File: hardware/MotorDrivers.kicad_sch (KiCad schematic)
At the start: 8 parts, among them M1 M1_CONN, M2 M2_CONN, M3 M3_CONN, M4 M4_CONN, U103 STSPIN240, U104 STSPIN240, U105 STSPIN240, U106 STSPIN240

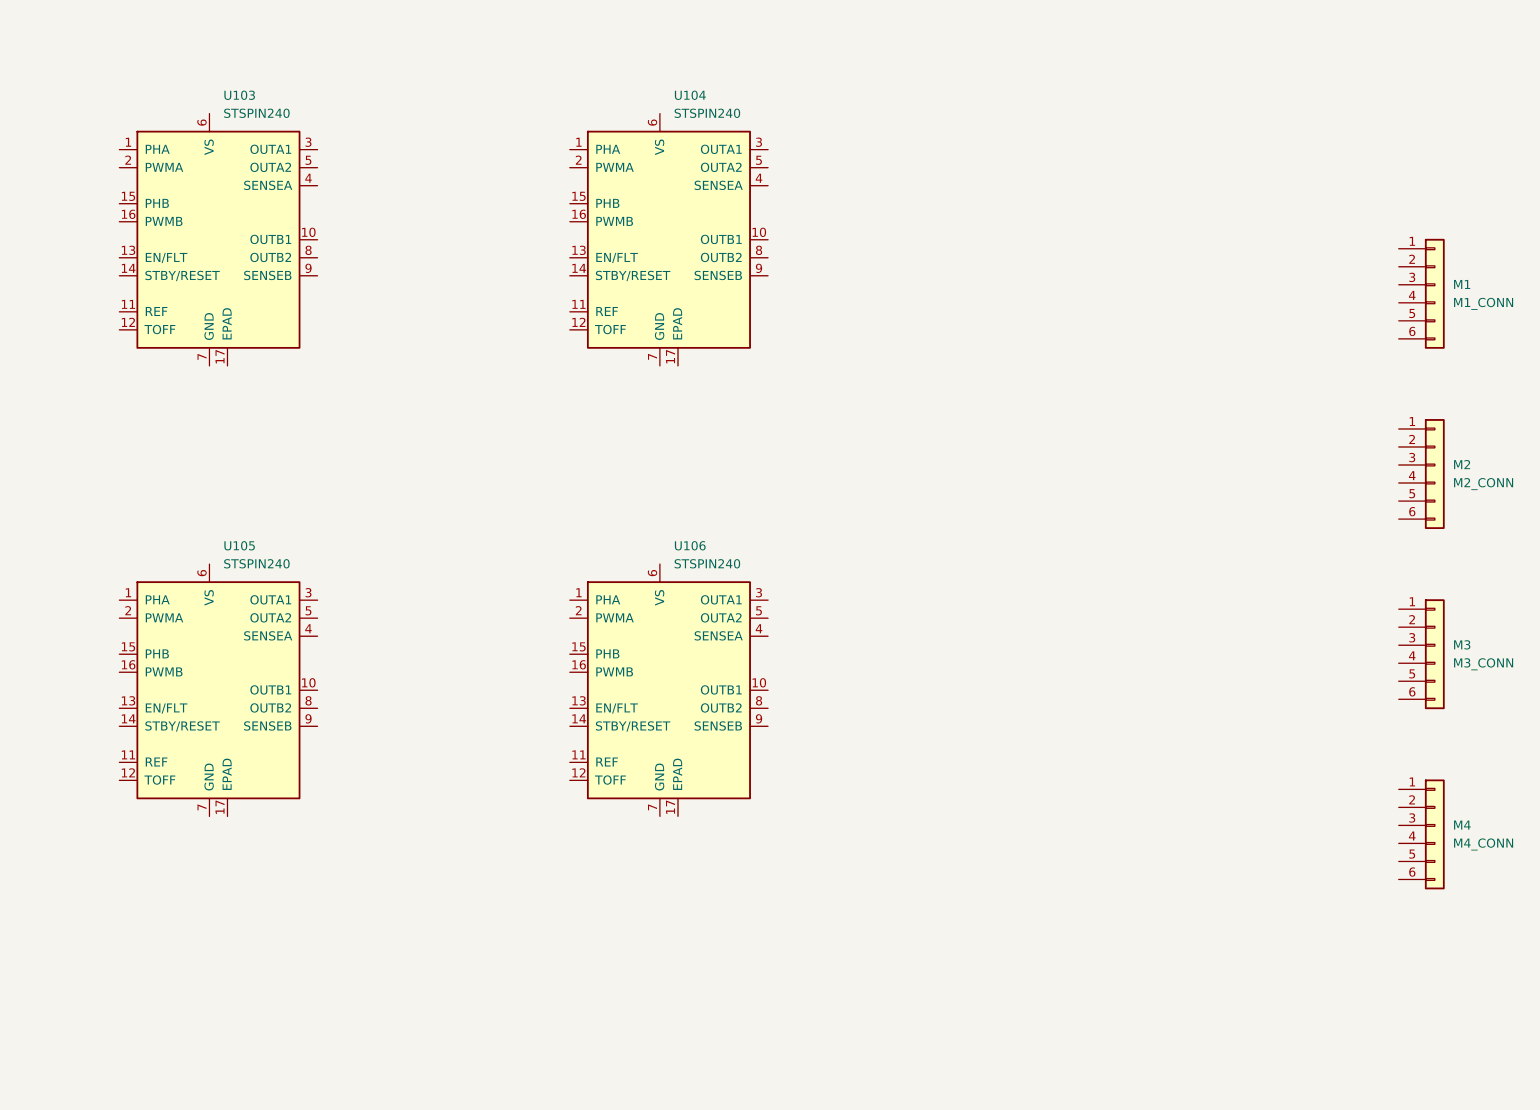
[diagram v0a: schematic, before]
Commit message: asdf
Signed-off-by: Connor Rigby <connorr@hey.com>
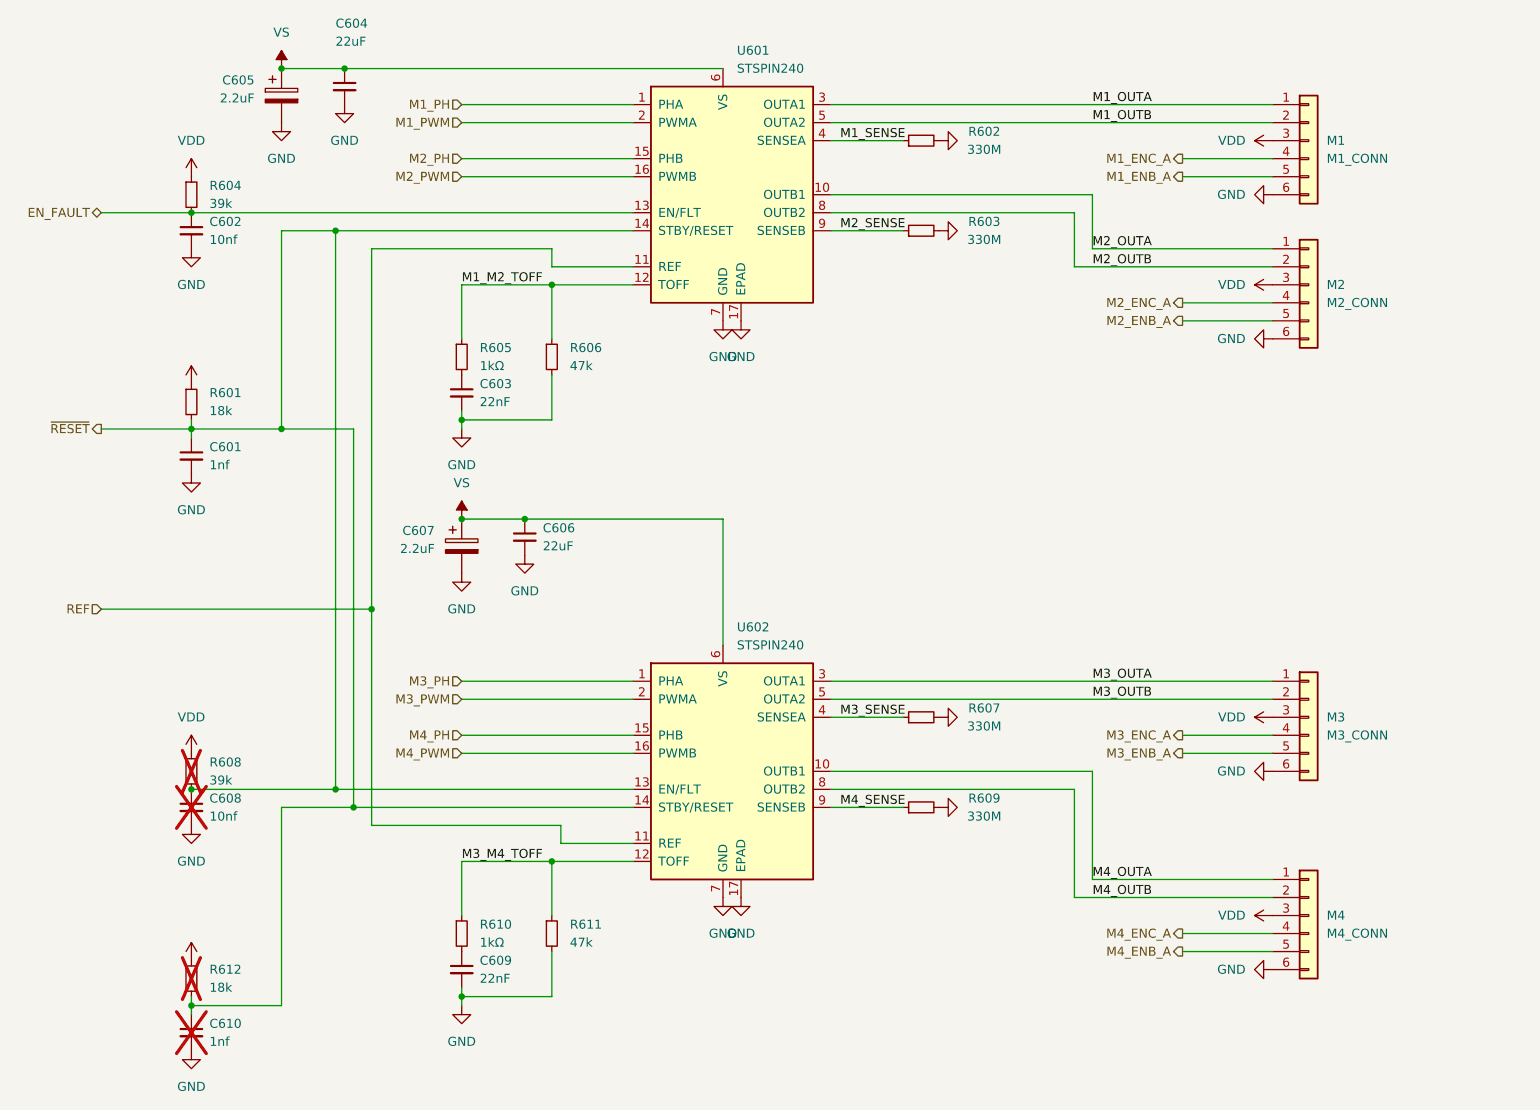
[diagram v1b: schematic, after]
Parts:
- removed U103, U104, U105, U106: STSPIN240, Package_DFN_QFN:VQFN-16-1EP_3x3mm_P0.5mm_EP1.8x1.8mm, symbol Driver_Motor:STSPIN240
- added C601, C610: C_0402_1nf_X7R, Capacitor_SMD:C_0402_1005Metric, symbol LCSC_Capacitor:C_0402_1nf_X7R
- added C602, C608: C_0402_10n_C0G, Capacitor_SMD:C_0402_1005Metric, symbol LCSC_Capacitor:C_0402_10n_C0G
- added C603, C609: C_0402_DNP, Capacitor_SMD:C_0402_1005Metric, symbol LCSC_Capacitor:C_0402_DNP
- added C604, C606: C_805_DNP, Capacitor_SMD:C_0805_2012Metric, symbol LCSC_Capacitor:C_805_DNP
- added C605, C607: 2.2uF, Capacitor_SMD:CP_Elec_5x3, symbol Device:C_Polarized
- added R601, R612: 18k, Resistor_SMD:R_0402_1005Metric, symbol LCSC_Resistor:R_0402_DNP
- added R602, R603, R607, R609: 330M, Resistor_SMD:R_0805_2012Metric, symbol Device:R_Small
- added R604, R608: 39k, Resistor_SMD:R_0402_1005Metric, symbol LCSC_Resistor:R_0402_DNP
- added R605, R610: R_0402_1k, Resistor_SMD:R_0402_1005Metric, symbol LCSC_Resistor:R_0402_1k
- added R606, R611: 47k, Resistor_SMD:R_0402_1005Metric, symbol LCSC_Resistor:R_0402_DNP
- added U601, U602: STSPIN240, Package_DFN_QFN:VQFN-16-1EP_3x3mm_P0.5mm_EP1.8x1.8mm, symbol Driver_Motor:STSPIN240
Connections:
- net M1_OUTA: now reaches M1.1 (Pin_1)
- net M1_OUTA: now also U601.3 (OUTA1)
- net M1_OUTB: now reaches M1.2 (Pin_2)
- net M1_OUTB: now also U601.5 (OUTA2)
- net VDD: now reaches M1.3 (Pin_3)
- net VDD: now also M2.3 (Pin_3), M3.3 (Pin_3), M4.3 (Pin_3), R601.1, R604.1, R608.1, R612.1
- net M1_ENC_A: now reaches M1.4 (Pin_4)
- net M1_ENB_A: now reaches M1.5 (Pin_5)
- net GND: now reaches M1.6 (Pin_6)
- net GND: now also M2.6 (Pin_6), M3.6 (Pin_6), M4.6 (Pin_6), C601.2, C602.2, C603.2, C604.2, C605.2, C606.2, C607.2, C608.2, C609.2, C610.2, R602.2, R603.2, R606.2, R607.2, R609.2, R611.2, U601.17 (EPAD), U601.7 (GND), U602.17 (EPAD), U602.7 (GND)
- net M4_OUTA: now reaches M4.1 (Pin_1)
- net M4_OUTA: now also U602.10 (OUTB1)
- net M4_OUTB: now reaches M4.2 (Pin_2)
- net M4_OUTB: now also U602.8 (OUTB2)
- net M4_ENC_A: now reaches M4.4 (Pin_4)
- net M4_ENB_A: now reaches M4.5 (Pin_5)
- net M2_OUTA: now reaches M2.1 (Pin_1)
- net M2_OUTA: now also U601.10 (OUTB1)
- net M2_OUTB: now reaches M2.2 (Pin_2)
- net M2_OUTB: now also U601.8 (OUTB2)
- net M2_ENC_A: now reaches M2.4 (Pin_4)
- net M2_ENB_A: now reaches M2.5 (Pin_5)
- net M3_OUTA: now reaches M3.1 (Pin_1)
- net M3_OUTA: now also U602.3 (OUTA1)
- net M3_OUTB: now reaches M3.2 (Pin_2)
- net M3_OUTB: now also U602.5 (OUTA2)
- net M3_ENC_A: now reaches M3.4 (Pin_4)
- net M3_ENB_A: now reaches M3.5 (Pin_5)
- new net: C603.1, R605.2
- new net: C609.1, R610.2
- new net EN_FAULT: C602.1, R604.2, U601.13 (EN/FLT)
- new net M1_M2_TOFF: R605.1, R606.1, U601.12 (TOFF)
- new net M1_PH: U601.1 (PHA)
- new net M1_PWM: U601.2 (PWMA)
- new net M1_SENSE: R602.1, U601.4 (SENSEA)
- new net M2_PH: U601.15 (PHB)
- new net M2_PWM: U601.16 (PWMB)
- new net M2_SENSE: R603.1, U601.9 (SENSEB)
- new net M3_M4_TOFF: R610.1, R611.1, U602.12 (TOFF)
- new net M3_PH: U602.1 (PHA)
- new net M3_PWM: U602.2 (PWMA)
- new net M3_SENSE: R607.1, U602.4 (SENSEA)
- new net M4_PH: U602.15 (PHB)
- new net M4_PWM: U602.16 (PWMB)
- new net M4_SENSE: R609.1, U602.9 (SENSEB)
- new net REF: U601.11 (REF), U602.11 (REF)
- new net VS: C604.1, C605.1, C606.1, C607.1, U601.6 (VS), U602.6 (VS)
- new net ~{RESET}: C601.1, C608.1, C610.1, R601.2, R608.2, R612.2, U601.14 (STBY/RESET), U602.13 (EN/FLT), U602.14 (STBY/RESET)
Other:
- moved on the sheet: M1, M2, M3, M4
